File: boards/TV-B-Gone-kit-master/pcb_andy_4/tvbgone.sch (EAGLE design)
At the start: 34 parts, among them U1 ATMEGA328P, Y1 18MHZ

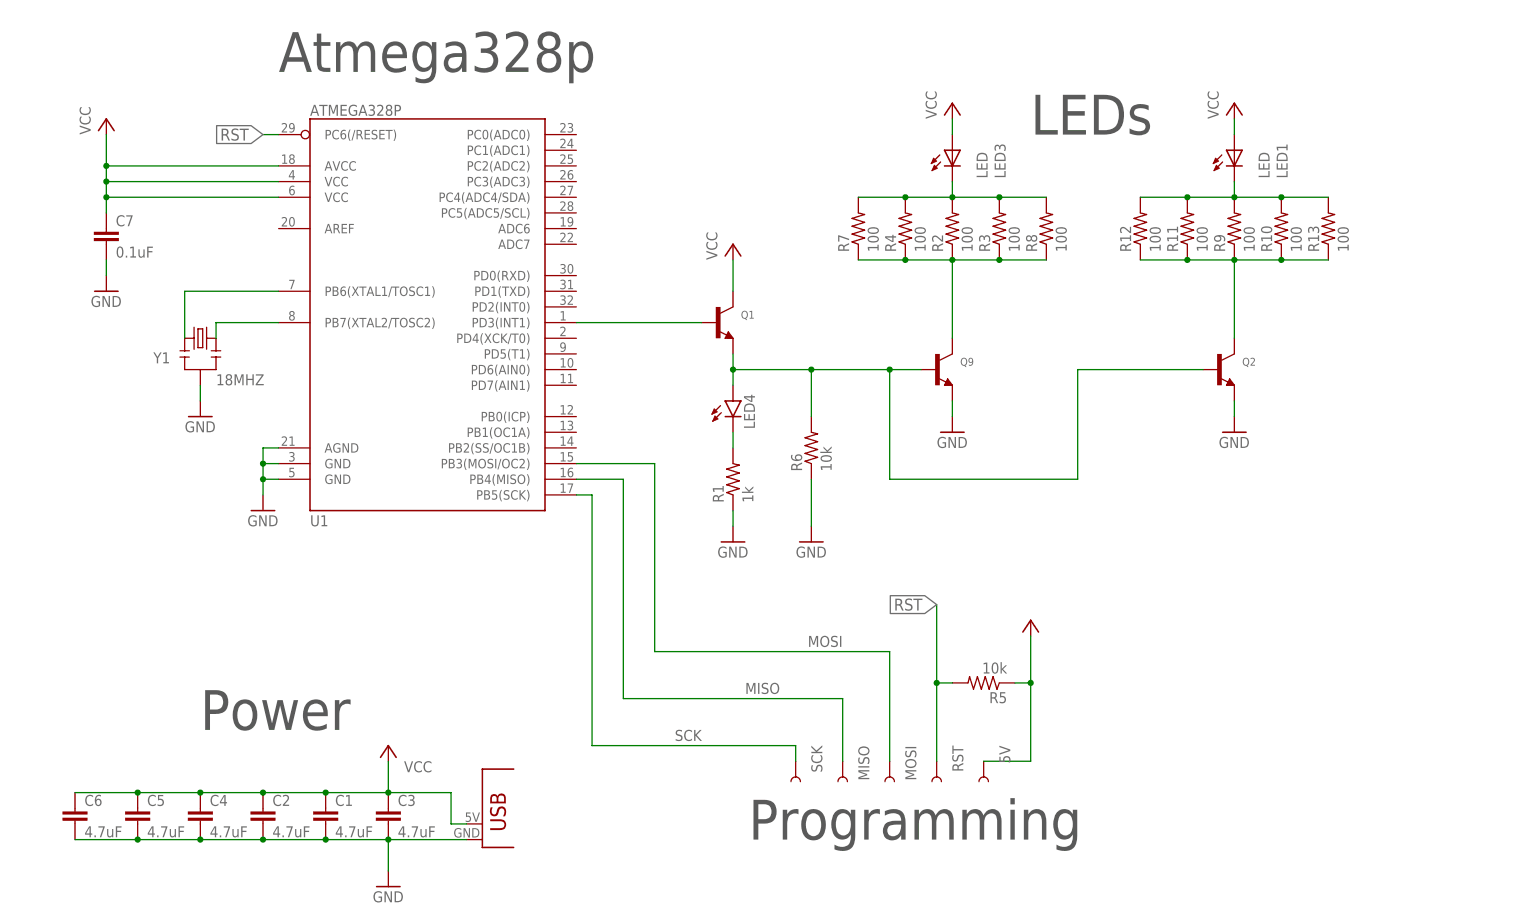
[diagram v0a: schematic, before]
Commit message: about to populate panels at ITP
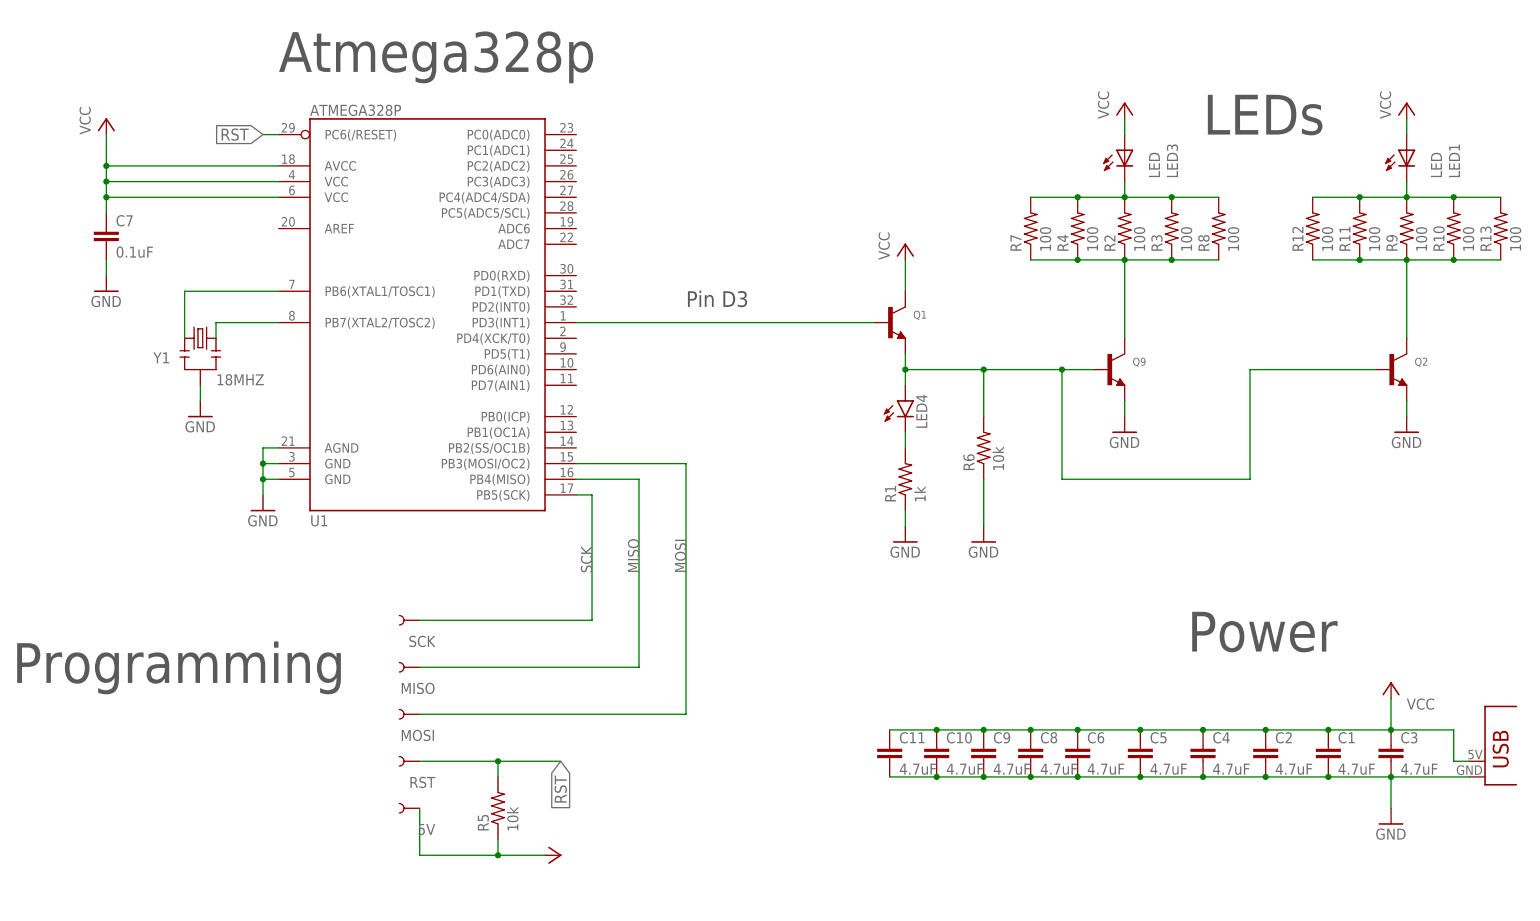
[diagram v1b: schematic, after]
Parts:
- added C10, C11, C8, C9: 4.7uF, homemade-hardware:CAP0603-CAP
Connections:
- net GND: now also C10.2, C11.2, C8.2, C9.2
- net VCC: now also C10.1, C11.1, C8.1, C9.1
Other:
- note added: "Pin D3"
- moved on the sheet: 5V, C1, C2, C3, C4, C5, C6, LED1, LED3, LED4, MISO, MOSI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
